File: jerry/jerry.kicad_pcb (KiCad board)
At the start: 2 copper layers, 7 parts, among them U1 RASPBERRY_PI_4B_4GB

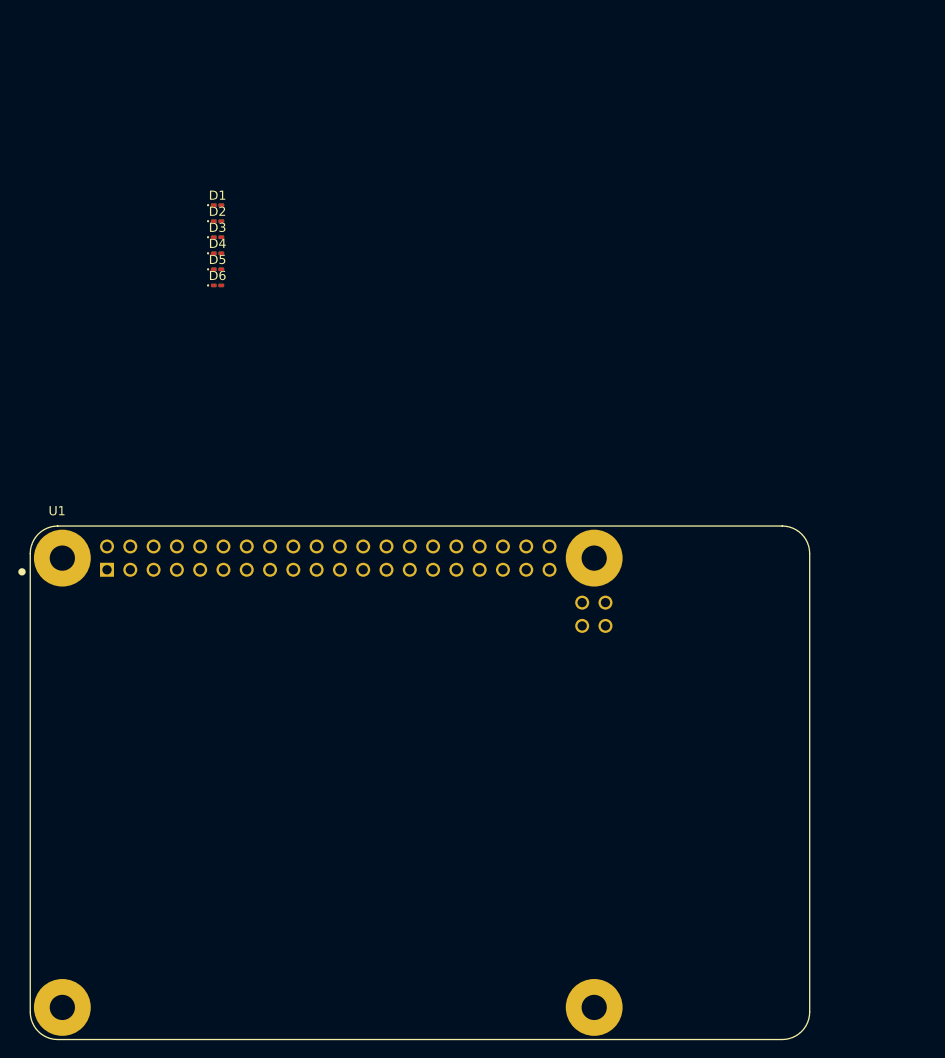
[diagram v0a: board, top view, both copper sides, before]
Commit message: Finished PCB
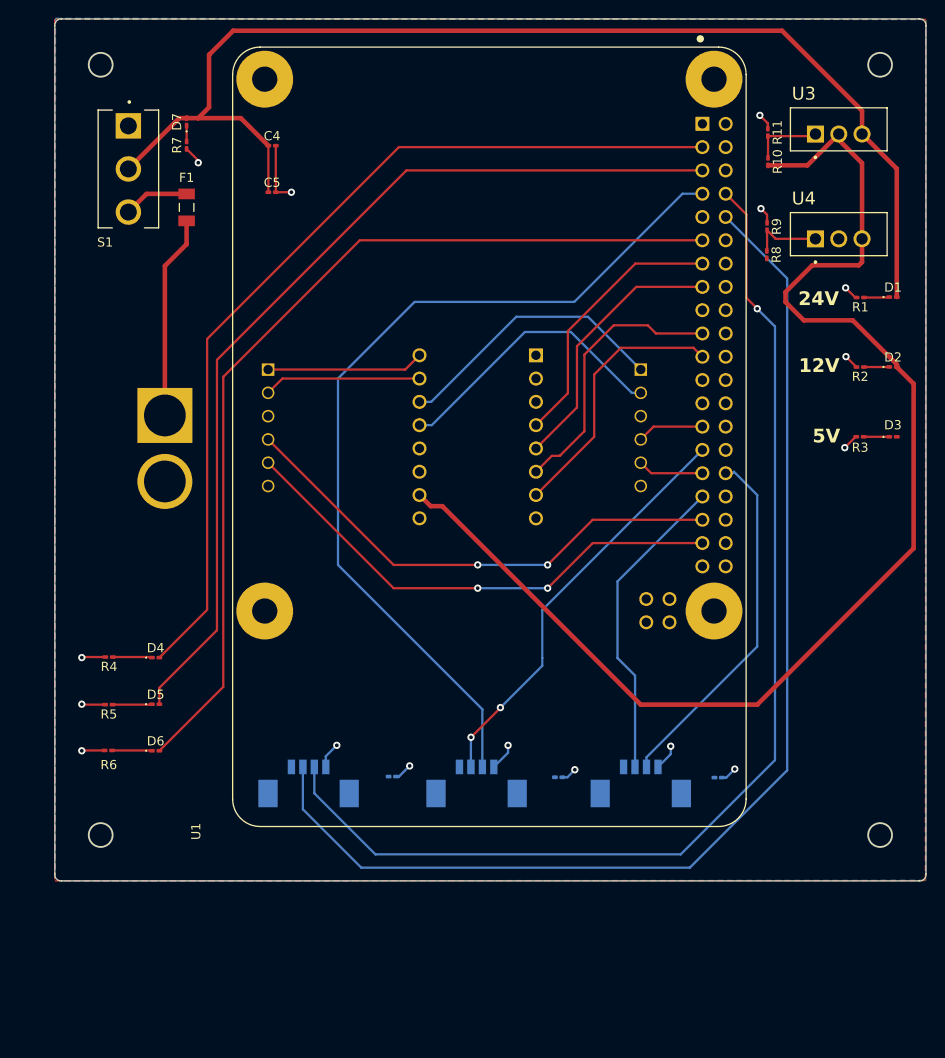
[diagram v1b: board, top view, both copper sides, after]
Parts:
- added C1: .1uF, Capacitor_SMD:C_0201_0603Metric_Pad0.64x0.40mm_HandSolder, B.Cu at (61.8, 152.6)
- added C2: .1uF, Capacitor_SMD:C_0201_0603Metric_Pad0.64x0.40mm_HandSolder, B.Cu at (79.9, 152.7)
- added C3: .1uF, Capacitor_SMD:C_0201_0603Metric_Pad0.64x0.40mm_HandSolder, B.Cu at (97.3, 152.7)
- added C4: 1uF, Capacitor_SMD:C_0201_0603Metric_Pad0.64x0.40mm_HandSolder, F.Cu at (48.7, 83.8)
- added C5: 10uF, Capacitor_SMD:C_0201_0603Metric_Pad0.64x0.40mm_HandSolder, F.Cu at (48.7, 88.9)
- added D7: LED, Diode_SMD:D_0201_0603Metric_Pad0.64x0.40mm_HandSolder, F.Cu at (39.4, 81.2)
- added F1: Fuse, jerry:FUSC3215X83N, F.Cu at (39.4, 90.5)
- added J1: 0532610471, jerry:MOLEX_0532610471, B.Cu at (52.7, 151.6)
- added J2: 0532610471, jerry:MOLEX_0532610471, B.Cu at (71.0, 151.6)
- added J3: 0532610471, jerry:MOLEX_0532610471, B.Cu at (88.9, 151.6)
- added J4: XT60-M, jerry:AMASS_XT60-M, B.Cu at (37.0, 116.8)
- added J7: TSW-106-06-F-S-LL, jerry:SAMTEC_TSW-106-06-F-S-LL, B.Cu at (48.3, 108.2)
- added J8: TSW-106-06-F-S-LL, jerry:SAMTEC_TSW-106-06-F-S-LL, B.Cu at (88.9, 108.2)
- added R1: 2k, Resistor_SMD:R_0201_0603Metric_Pad0.64x0.40mm_HandSolder, F.Cu at (112.8, 100.4)
- added R10: 2k, Resistor_SMD:R_0201_0603Metric_Pad0.64x0.40mm_HandSolder, F.Cu at (102.8, 85.6)
- added R11: 2k, Resistor_SMD:R_0201_0603Metric_Pad0.64x0.40mm_HandSolder, F.Cu at (102.8, 82.4)
- added R2: 1k, Resistor_SMD:R_0201_0603Metric_Pad0.64x0.40mm_HandSolder, F.Cu at (112.8, 108.0)
- added R3: 330, Resistor_SMD:R_0201_0603Metric_Pad0.64x0.40mm_HandSolder, F.Cu at (112.8, 115.6)
- added R4: 1k, Resistor_SMD:R_0201_0603Metric_Pad0.64x0.40mm_HandSolder, F.Cu at (30.9, 139.6)
- added R5: 1k, Resistor_SMD:R_0201_0603Metric_Pad0.64x0.40mm_HandSolder, F.Cu at (30.9, 144.8)
- added R6: 1k, Resistor_SMD:R_0201_0603Metric_Pad0.64x0.40mm_HandSolder, F.Cu at (30.8, 149.8)
- added R7: 2k, Resistor_SMD:R_0201_0603Metric_Pad0.64x0.40mm_HandSolder, F.Cu at (39.4, 83.8)
- added R8: 2k, Resistor_SMD:R_0201_0603Metric_Pad0.64x0.40mm_HandSolder, F.Cu at (102.6, 95.7)
- added R9: 2k, Resistor_SMD:R_0201_0603Metric_Pad0.64x0.40mm_HandSolder, F.Cu at (102.7, 92.6)
- added S1: 500SSP1S2M2QEA, jerry:SW_500SSP1S2M2QEA, F.Cu at (33.0, 86.4)
- added U2: A4988_STEPPER_MOTOR_DRIVER_CARRIER, jerry:MODULE_A4988_STEPPER_MOTOR_DRIVER_CARRIER, B.Cu at (71.1, 115.6)
- added U3: LM338T, jerry:TO254P1054X470X1955-3, F.Cu at (110.5, 82.5)
- added U4: LM338T, jerry:TO254P1054X470X1955-3, F.Cu at (110.5, 94.0)
- moved D3 76.8 mm to (116.4, 115.6)
- moved D2 75.4 mm to (116.4, 108.0)
- moved D1 74.3 mm to (116.4, 100.3)
- moved D6 51.2 mm to (36.0, 149.8)
- moved D5 47.9 mm to (36.0, 144.7)
- moved D4 44.6 mm to (36.0, 139.7)
- moved U1 38.5 mm to (72.4, 115.6), turned to -90 degrees
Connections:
- net Net-(U1-GND-Pad14) renamed GND
- D1 pad 1: unconnected-(D1-K-Pad1) -> Net-(D1-K)
- D1 pad 2: unconnected-(D1-A-Pad2) -> +24V
- D2 pad 1: unconnected-(D2-K-Pad1) -> Net-(D2-K)
- D2 pad 2: unconnected-(D2-A-Pad2) -> +12V
- D3 pad 1: unconnected-(D3-K-Pad1) -> Net-(D3-K)
- D3 pad 2: unconnected-(D3-A-Pad2) -> +5V
- D4 pad 1: unconnected-(D4-K-Pad1) -> Net-(D4-K)
- D4 pad 2: unconnected-(D4-A-Pad2) -> /LEDInd1
- D5 pad 1: unconnected-(D5-K-Pad1) -> Net-(D5-K)
- D5 pad 2: unconnected-(D5-A-Pad2) -> /LEDInd2
- D6 pad 1: unconnected-(D6-K-Pad1) -> Net-(D6-K)
- D6 pad 2: unconnected-(D6-A-Pad2) -> /LEDInd3
- U1 pad 10: unconnected-(U1-GPIO15/RXD0-Pad10) -> /TFMINITX1
- U1 pad 11: unconnected-(U1-GPIO17/GPIO_GEN0-Pad11) -> /LEDInd3
- U1 pad 13: unconnected-(U1-GPIO27/GPIO_GEN2-Pad13) -> /IN1
- U1 pad 15: unconnected-(U1-GPIO22/GPIO_GEN3-Pad15) -> /IN2
- U1 pad 19: unconnected-(U1-GPIO10/SPI_MOSI-Pad19) -> /IN3
- U1 pad 2: Net-(U1-5V-Pad2) -> +5V
- U1 pad 21: unconnected-(U1-GPIO9/SPI_MISO-Pad21) -> /IN4
- U1 pad 27: unconnected-(U1-ID_SD-Pad27) -> /OUTA_B
- U1 pad 29: unconnected-(U1-GPIO5-Pad29) -> /TFMINITX2
- U1 pad 3: unconnected-(U1-GPIO2/SDA1-Pad3) -> /LEDInd1
- U1 pad 31: unconnected-(U1-GPIO6-Pad31) -> /OUTB_B
- U1 pad 32: unconnected-(U1-GPIO12-Pad32) -> /TFMINIRX3
- U1 pad 33: unconnected-(U1-GPIO13-Pad33) -> /TFMINITX3
- U1 pad 35: unconnected-(U1-GPIO19-Pad35) -> /OUTA_A
- U1 pad 37: unconnected-(U1-GPIO26-Pad37) -> /OUTB_A
- U1 pad 4: Net-(U1-5V-Pad2) -> +5V
- U1 pad 5: unconnected-(U1-GPIO3/SCL1-Pad5) -> /LEDInd2
- U1 pad 7: unconnected-(U1-GPIO4/GPIO_GCKL-Pad7) -> /TFMINIRX2
- U1 pad 8: unconnected-(U1-GPIO14/TXD0-Pad8) -> /TFMINIRX1
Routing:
- net +12V: track 0.00 -> 141.1 mm
- net +24V: track 0.00 -> 129.1 mm
- net /TFMINITX1: track 0.00 -> 127.6 mm
- net /TFMINIRX1: track 0.00 -> 124.1 mm, vias 0 -> 1
- net /LEDInd3: track 0.00 -> 102.1 mm
- net /LEDInd2: track 0.00 -> 101.6 mm
- net /LEDInd1: track 0.00 -> 99.6 mm
- net /TFMINIRX2: track 0.00 -> 97.0 mm
- net /OUTB_A: track 0.00 -> 55.1 mm, vias 0 -> 2
- net /OUTA_A: track 0.00 -> 55.1 mm, vias 0 -> 2
- net /TFMINITX2: track 0.00 -> 45.1 mm, vias 0 -> 2
- net /TFMINIRX3: track 0.00 -> 39.2 mm
- net /TFMINITX3: track 0.00 -> 34.1 mm
- net /M2B: track 0.00 -> 31.1 mm
- net /M1B: track 0.00 -> 30.4 mm
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- added copper zone on F.Cu, net +5V
- added copper zone on B.Cu, net GND
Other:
- board outline added: 95 x 94 mm
- board text added: "12V"
- board text added: "24V"
- board text added: "5V"
